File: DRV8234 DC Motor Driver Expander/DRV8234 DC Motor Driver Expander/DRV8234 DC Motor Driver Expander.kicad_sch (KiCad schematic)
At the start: 20 parts, among them IC1 DRV8234RTER, J1 POWER, J2 CNTRL_IN, J3 CNTRL_OUT, J4 I2C, J5 MOTOR

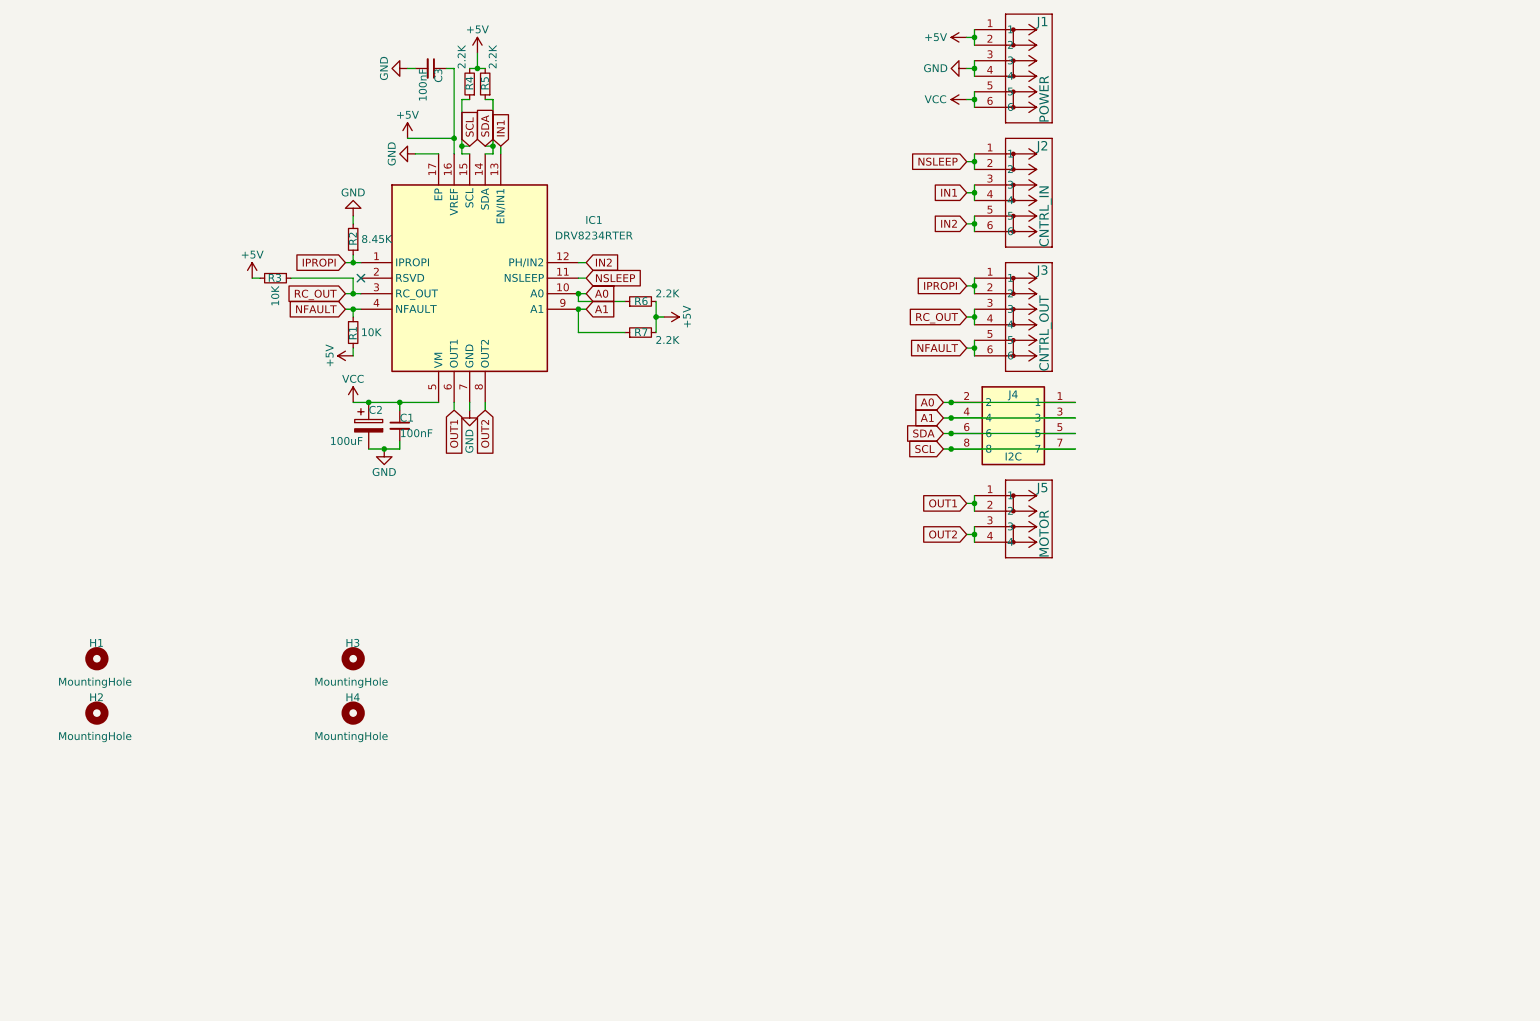
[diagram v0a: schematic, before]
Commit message: V2
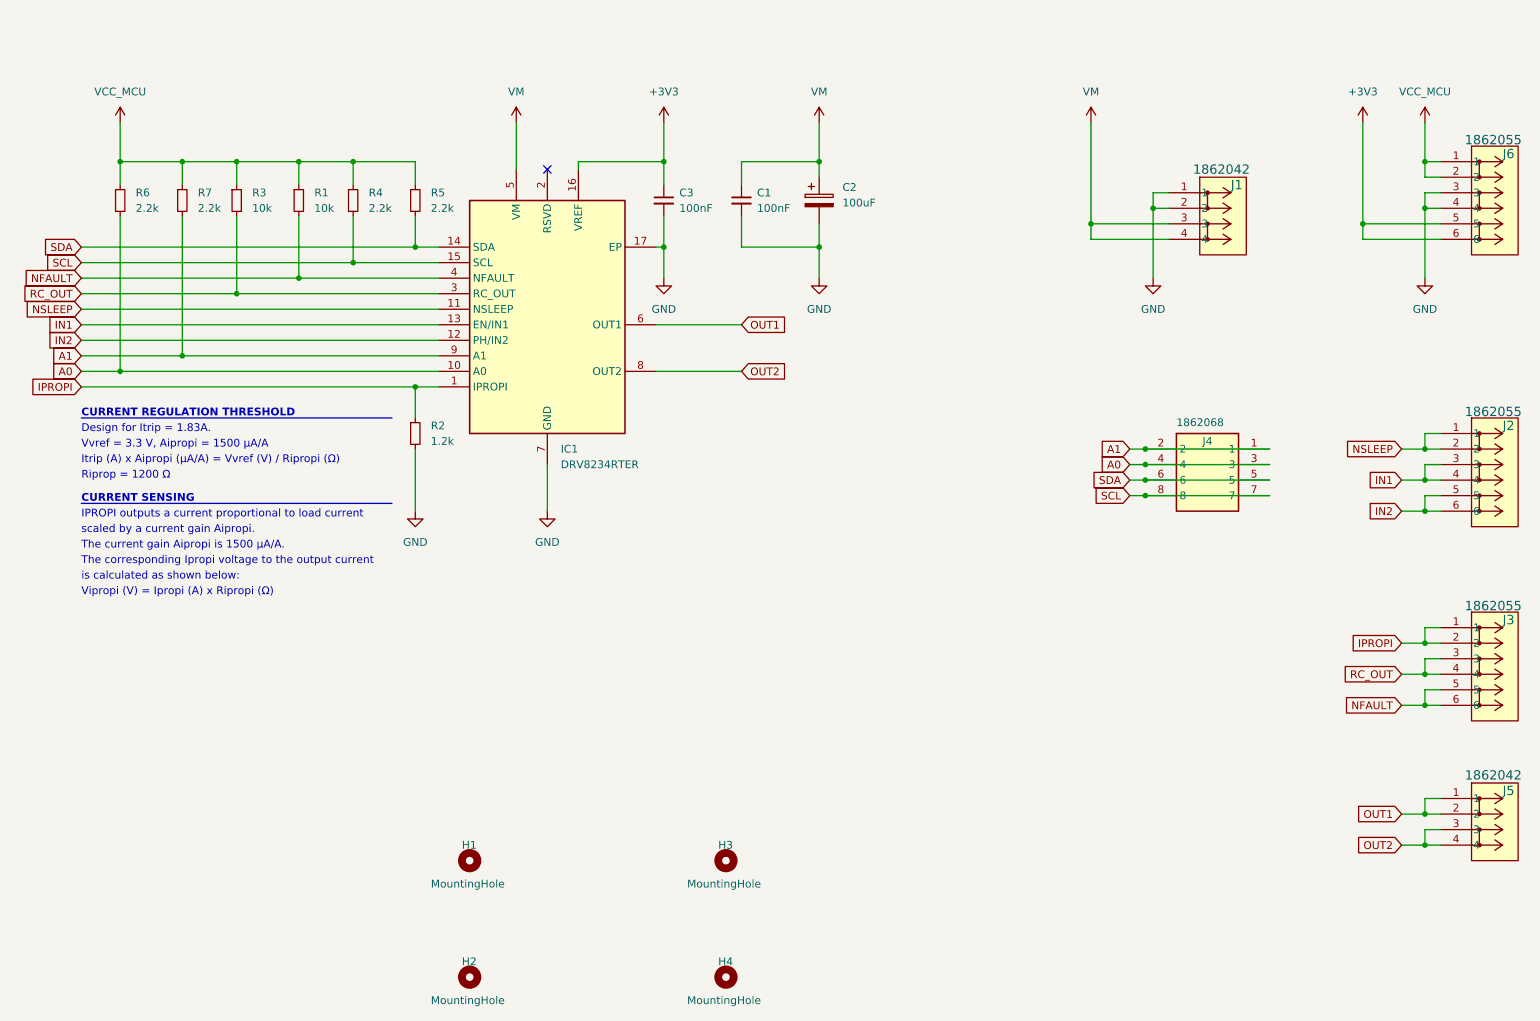
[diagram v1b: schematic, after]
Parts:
- removed J1: POWER, 1862055 Footprint:CONN_1862055, symbol 1862055:1862055
- added J1: 1862042, PCB Footprints:1862042, symbol Schematic Symbols:1862042
- added J6: 1862055, PCB Footprints:1862055, symbol Schematic Symbols:1862055
- C1, C3: footprint Capacitor_SMD:C_1206_3216Metric_Pad1.33x1.80mm_HandSolder -> Capacitor_SMD:C_0805_2012Metric; Manufacturer_Name (none) -> Aillen; Manufacturer_Part_Number (none) -> 0805B104K101CC
- C2: Manufacturer_Name (none) -> Nichicon; Manufacturer_Part_Number (none) -> UWT1H101MNL1GS
- IC1: footprint DRV8234 Footprint:QFN50P300X300X80-17N-D -> PCB Footprints:DRV8234RTER; symbol DRV8234:DRV8234RTER -> Schematic Symbols:DRV8234RTER; Height 0.8 -> (none)
- J2: value CNTRL_IN -> 1862055; footprint 1862055 Footprint:CONN_1862055 -> PCB Footprints:1862055; symbol 1862055:1862055 -> Schematic Symbols:1862055; Manufacturer_Name (none) -> Phoenix Contact; Manufacturer_Part_Number (none) -> 1862055
- J3: value CNTRL_OUT -> 1862055; footprint 1862055 Footprint:CONN_1862055 -> PCB Footprints:1862055; symbol 1862055:1862055 -> Schematic Symbols:1862055; Manufacturer_Name (none) -> Phoenix Contact; Manufacturer_Part_Number (none) -> 1862055
- J4: value I2C -> 1862068; footprint 1862068 Footprint:1862068 -> PCB Footprints:1862068; symbol 1862068:1862068 -> Schematic Symbols:1862068; Height 10.2 -> (none); Mouser Part Number 651-1862068 -> (none); Mouser Price/Stock https://www.mouser.co.uk/ProductDetail/Phoenix-Contact/1862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 -> (none)
- J5: value MOTOR -> 1862042; footprint 1862042 Footprint:CONN_1862042 -> PCB Footprints:1862042; symbol 1862042:1862042 -> Schematic Symbols:1862042; Manufacturer_Name (none) -> Phoenix Contact; Manufacturer_Part_Number (none) -> 1862042
- R1, R3: value 10K -> 10k; footprint Resistor_SMD:R_0805_2012Metric_Pad1.20x1.40mm_HandSolder -> Resistor_SMD:R_0805_2012Metric; Manufacturer_Name (none) -> YAGEO; Manufacturer_Part_Number (none) -> RC0805FR-0710KL
- R2: value 8.45K -> 1.2k; footprint Resistor_SMD:R_0805_2012Metric_Pad1.20x1.40mm_HandSolder -> Resistor_SMD:R_0805_2012Metric; Manufacturer_Name (none) -> TE Connectivity Passive Product; Manufacturer_Part_Number (none) -> CRG0805F1K2
- R4, R5, R6, R7: value 2.2K -> 2.2k; footprint Resistor_SMD:R_0805_2012Metric_Pad1.20x1.40mm_HandSolder -> Resistor_SMD:R_0805_2012Metric; Manufacturer_Name (none) -> YAGEO; Manufacturer_Part_Number (none) -> RC0805FR-072K2L
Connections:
- net A0: now also J4.3, J4.4, R6.2; no longer J4.1, J4.2, R6.1
- net A1: now also J4.1, J4.2, R7.2; no longer J4.3, J4.4, R7.1
- net GND: now also J1.1, J1.2, J6.3, J6.4
- net NFAULT: now also R1.2; no longer R1.1
- net RC_OUT: now also R3.2; no longer R3.1
- net SCL: now also R4.2; no longer R4.1
- net SDA: now also R5.2; no longer R5.1
- removed net +5V: C3.1, IC1.16 (VREF), R1.2, R3.2, R4.2, R5.2, R6.2, R7.2
- net VCC renamed VM
- net VM: now also J1.3, J1.4
- new net +3V3: C3.1, IC1.16 (VREF), J6.5, J6.6
- new net VCC_MCU: J6.1, J6.2, R1.1, R3.1, R4.1, R5.1, R6.1, R7.1
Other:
- note added: "CURRENT REGULATION THRESHOLD"
- note added: "CURRENT SENSING"
- note added: "Design for Itrip = 1.83A."
- note added: "IPROPI outputs a current proportional to load current"
- note added: "Itrip (A) x Aipropi (μA/A) = Vvref (V) / Ripropi (Ω)"
- note added: "Riprop = 1200 Ω"
- note added: "The corresponding Ipropi voltage to the output current"
- note added: "The current gain Aipropi is 1500 μA/A."
- note added: "Vipropi (V) = Ipropi (A) x Ripropi (Ω)"
- note added: "Vvref = 3.3 V, Aipropi = 1500 μA/A"
- note added: "is calculated as shown below:"
- note added: "scaled by a current gain Aipropi."
- moved on the sheet: H1, H2, H3, H4, IC1, J4
